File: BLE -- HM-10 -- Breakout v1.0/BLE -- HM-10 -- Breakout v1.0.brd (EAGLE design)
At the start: 24 x 30.7 mm, 19 parts, among them U1 V_REG_LDOSMD

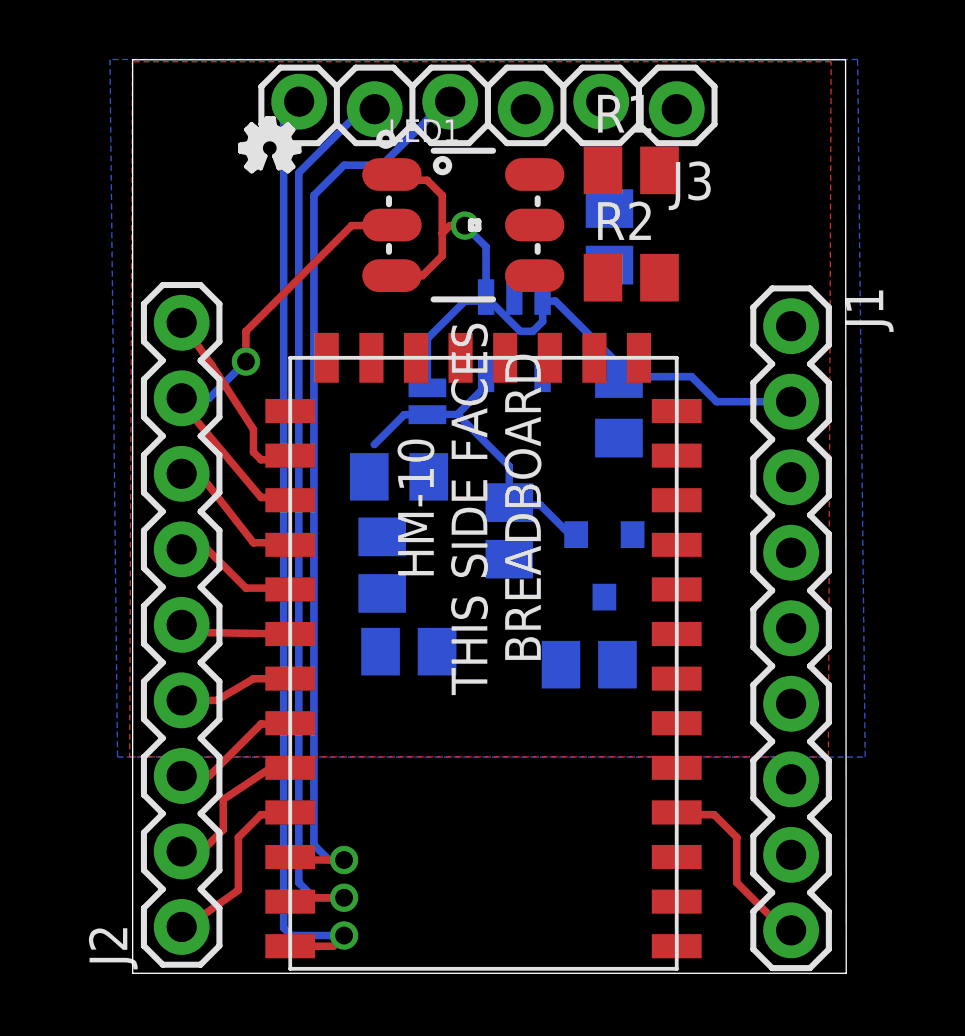
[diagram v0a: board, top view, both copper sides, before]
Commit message: Updating board
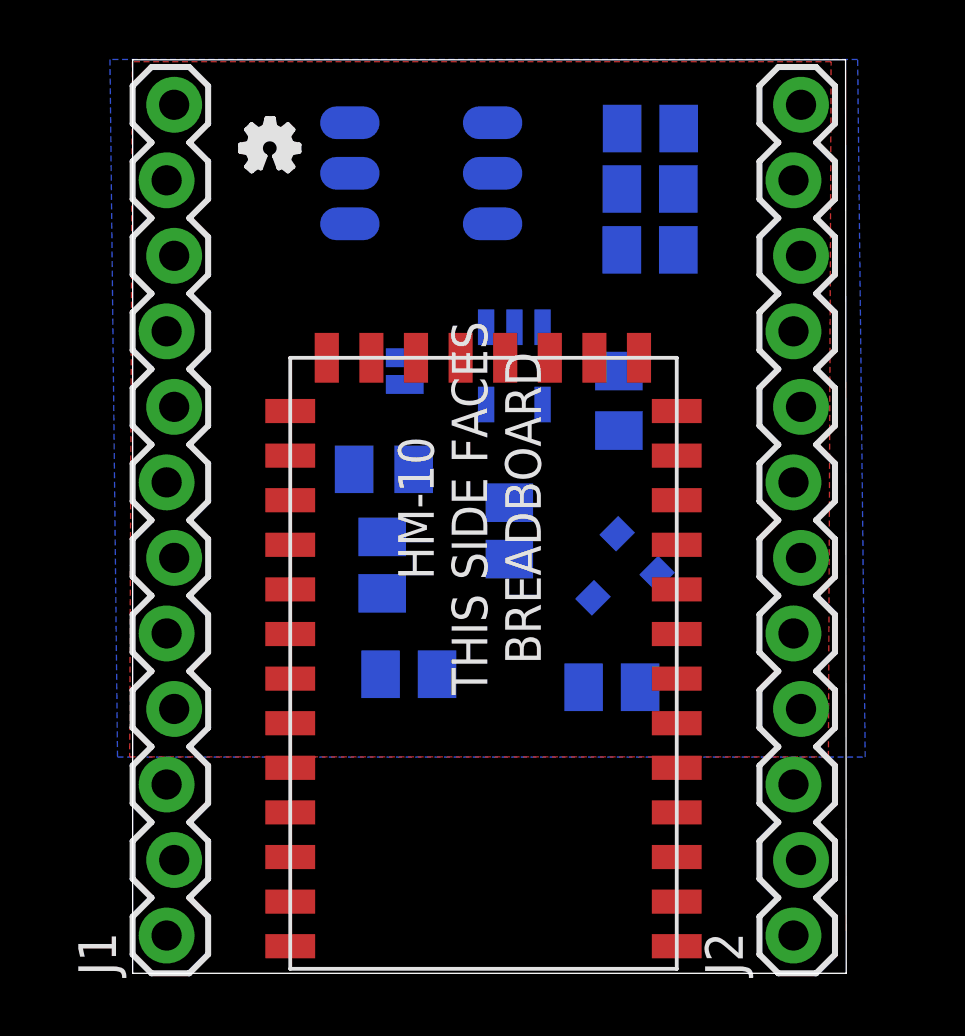
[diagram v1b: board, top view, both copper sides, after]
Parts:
- removed J3: (no value), SparkFun-Connectors:1X06_LOCK
- J1, J2: device SparkFun-Connectors:1X09 -> SparkFun-Connectors:1X12_LOCK
- moved J1 29.3 mm to (1.27, 1.27), turned to 90 degrees
- moved J2 20.7 mm to (22.4, 1.27)
- moved R2 5.06 mm to (17.4, 28.4), flipped to the bottom, turned to 180 degrees
- moved R1 2.75 mm to (17.4, 24.3), flipped to the bottom, turned to 180 degrees
- moved LED1 2.24 mm to (9.71, 26.9), flipped to the bottom, turned to 180 degrees
- moved R7 2.11 mm to (17.4, 26.4), turned to 180 degrees
- moved SJ1 1.27 mm to (9.15, 20.3)
- moved R5 1.08 mm to (16.1, 9.62)
- moved U1 1.02 mm to (12.8, 20.4)
- moved R4 0.76 mm to (9.29, 10.1)
- moved C2 0.57 mm to (8.45, 17.0)
- moved BSS138 0.53 mm to (16.3, 13.4), turned to 225 degrees
- moved C1 0.25 mm to (16.4, 19.3)
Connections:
- removed net PIO10: J3.5, U$1.PIO10
- removed net PIO9: J3.4, U$1.PIO9
- new net N$5: J1.2, U$1.PIO10
- new net N$6: J1.3, U$1.PIO9
- net 5V: now also J2.1; no longer J1.2
- net AIO0: now also J2.5; no longer J1.6
- net AIO1: now also J2.4; no longer J1.5
- net CTS: now also J2.9; no longer J3.1
- net GND: now also J2.10; no longer J1.1, J1.3
- net PIO0: now also J1.12; no longer J2.9
- net PIO1: now also J1.11; no longer J2.8
- net PIO11: now also J1.1; no longer J3.6
- net PIO2: now also J1.10; no longer J2.7
- net PIO3: now also J1.9; no longer J2.6
- net PIO4: now also J1.8; no longer J2.5
- net PIO5: now also J1.7; no longer J2.4
- net PIO6: now also J1.6; no longer J2.3
- net PIO7: now also J1.5; no longer J2.2
- net PIO8: now also J1.4; no longer J2.1
- net RESET: now also J2.3; no longer J1.4
- net RTS: now also J2.2; no longer J1.9
- net RX: now also J2.12; no longer J3.3
- net TX: now also J2.11; no longer J3.2
- net USBD+: now also J2.7; no longer J1.8
- net USBD-: now also J2.6; no longer J1.7
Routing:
- net PIO11: track 32.1 -> 0.00 mm, vias 1 -> 0
- net PIO10: track 30.9 -> 0.00 mm, vias 1 -> 0
- net PIO9: track 30.8 -> 0.00 mm, vias 1 -> 0
- net 5V: track 27.2 -> 0.00 mm, vias 1 -> 0
- net PIO1: track 15.4 -> 0.00 mm, vias 1 -> 0
- net 3_3V: track 11.3 -> 0.00 mm
- net PIO0: track 6.49 -> 0.00 mm
- net RTS: track 6.38 -> 0.00 mm
- net PIO8: track 6.17 -> 0.00 mm
- net PIO7: track 5.30 -> 0.00 mm
- net PIO2: track 4.81 -> 0.00 mm
- net PIO6: track 4.38 -> 0.00 mm
- net PIO3: track 4.21 -> 0.00 mm
- net PIO5: track 3.85 -> 0.00 mm
- net PIO4: track 3.72 -> 0.00 mm
